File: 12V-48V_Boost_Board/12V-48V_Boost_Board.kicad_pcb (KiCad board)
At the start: 2 copper layers, 80 x 64 mm, 35 parts, among them J1 12V Input, J2 Input Current Sensing, J3 Output Current Sensing, J4 48V Output, J5 Output Measuring, Q1 FDWS86068-F085

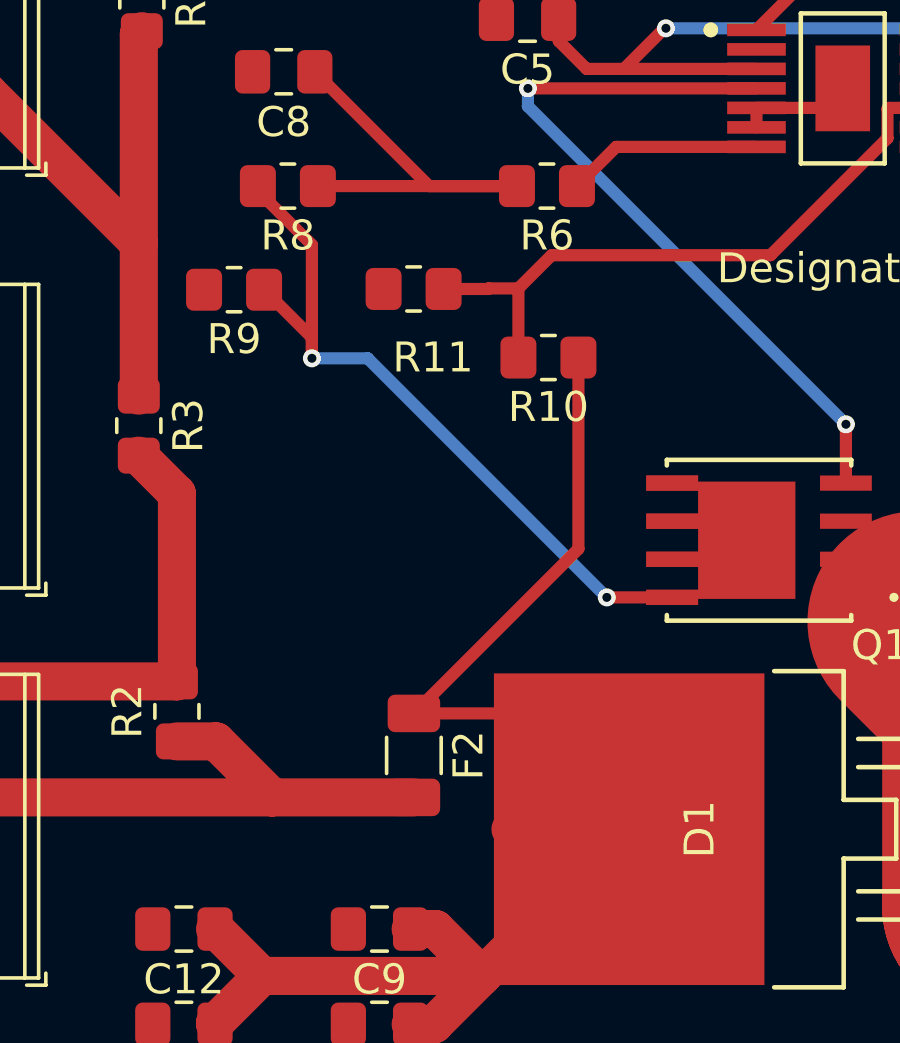
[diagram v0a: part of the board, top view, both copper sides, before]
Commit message: Minor touchup
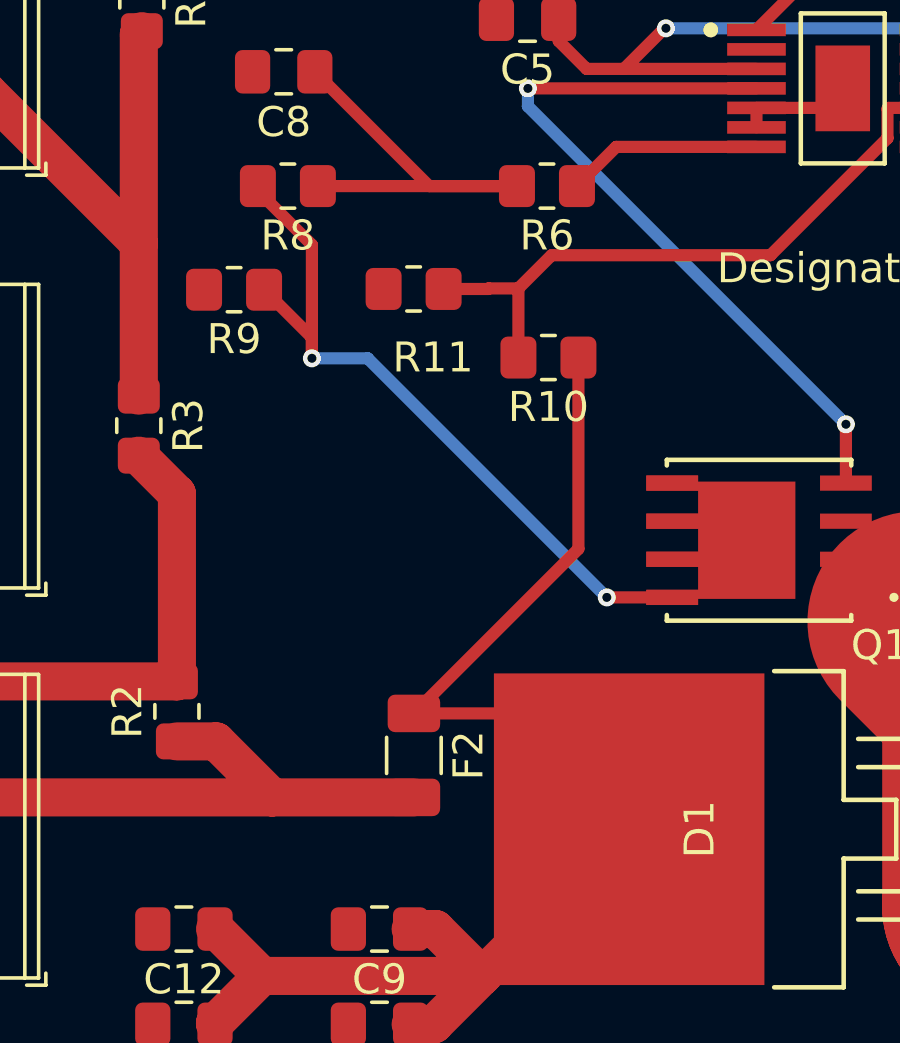
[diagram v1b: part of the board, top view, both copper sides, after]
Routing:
- net /Boost_Board_Chip/48V_OUTPUT: track 46.7 -> 42.3 mm
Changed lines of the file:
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@@
-	)
-	(segment
-		(start 154.7749 120.4976)
-		(end 154.7749 120.9851)
-		(width 1.27)
-		(layer "F.Cu")
-		(net 8)
 	)
 	(segment
@@
 	)
 	(segment
-		(start 154.7749 120.4976)
-		(end 150.8174 120.4976)
-		(width 1.27)
-		(layer "F.Cu")
-		(net 8)
-	)
-	(segment
 		(start 140.97 126.9514)
 		(end 142.5332 125.3882)
@@
 		(width 0.4064)
 		(layer "F.Cu")
-		(net 16)
-	)
-	(segment
-		(start 142.399 99.219)
-		(end 142.399 99.06)
-		(width 0.4064)
-		(layer "F.Cu")
